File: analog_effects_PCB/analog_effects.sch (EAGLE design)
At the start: 79 parts, among them J1 RN111PC, J2 SP-3533-02, J3 SAMTEC-SSQ-120-01-X-DJ, U1 TL082, U10 TS5A3359DCUT, U11 TS5A3359DCUT, U12 TS5A3359DCUT, U13 TS5A3359DCUT, U14 TS5A3359DCUT, U2 AD5241BRZ1M, U4 AD5241BRZ100, U7 AD5258BRMZ1-R7, U8 AD5241BRZ1M, U9 TS5A3359DCUT

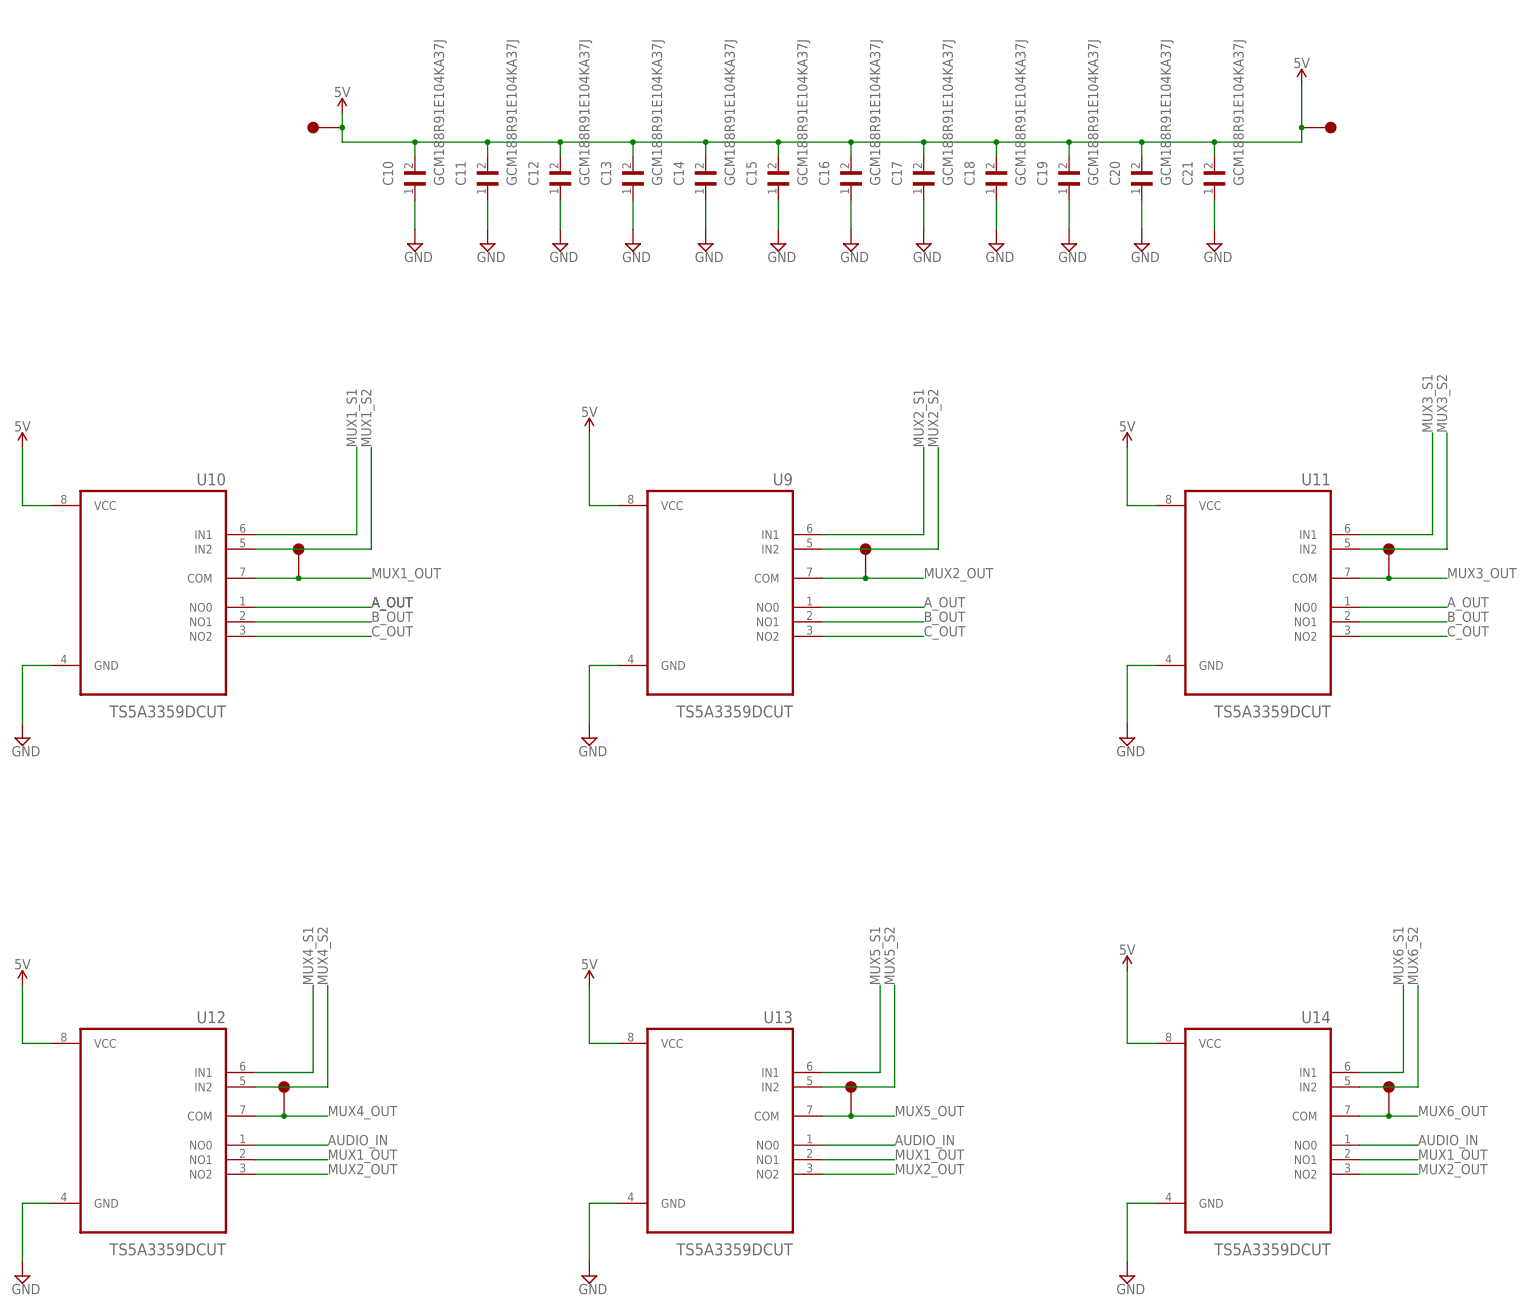
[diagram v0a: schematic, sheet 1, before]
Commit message: Adding all files that were needed, Capstone is completed and it worked
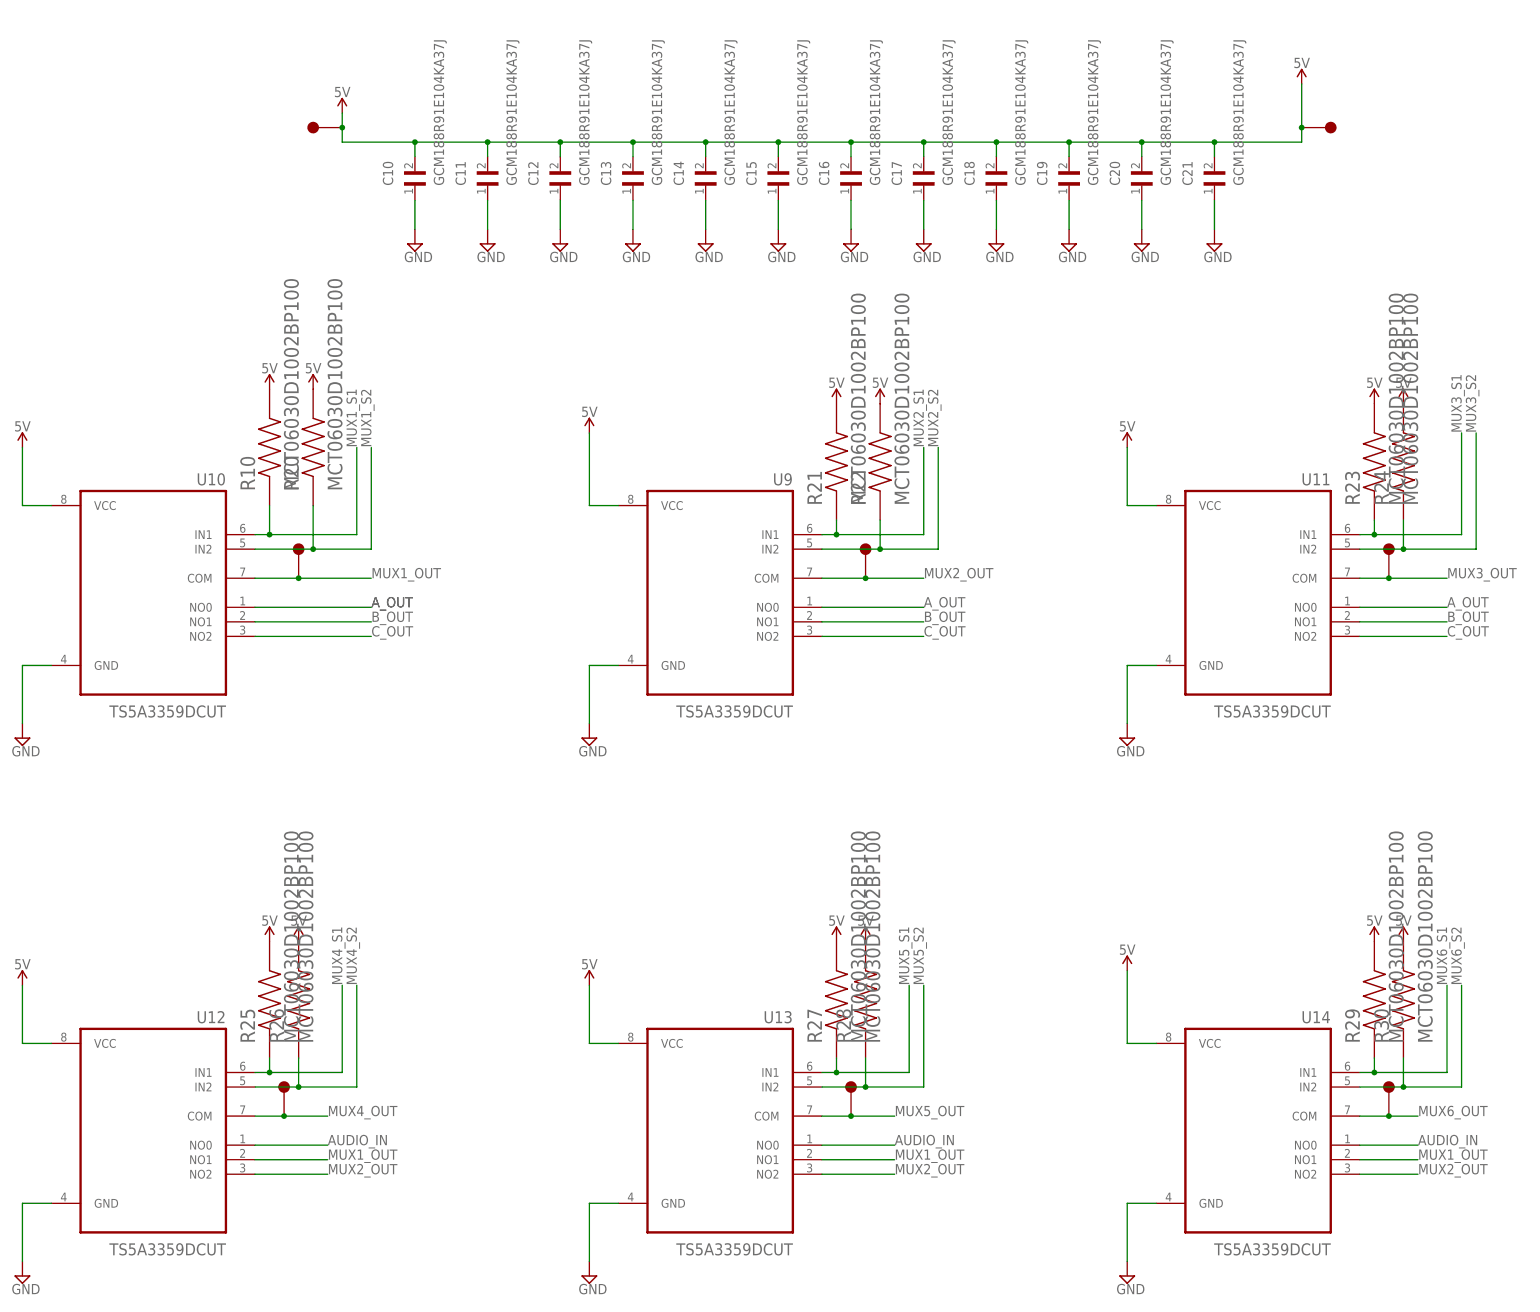
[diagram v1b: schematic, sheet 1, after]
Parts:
- removed BT1, BT2: BC9VPC, BC9VPC:BC9VPC
- removed J2: SP-3533-02, SP-3533-02:SP-3533-02
- added J4: SJ-3523-SMT-TR, SJ-3523-SMT-TR:SJ-3523-SMT-TR
- added R10, R20, R21, R22, R23, R24, R25, R26, R27, R28, R29, R30: MCT06030D1002BP100, MCT06030D1002BP100:MCT06030D1002BP100
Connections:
- removed net N$11: BT2.-, R17.2, R19.2, TP9.TP
- new net 9V_N: C4.2, C7.2, R17.2, R19.2, R5.1, TP2.TP, TP9.TP
- net 5V: now also R10.2, R20.2, R21.2, R22.2, R23.2, R24.2, R25.2, R26.2, R27.2, R28.2, R29.2, R30.2
- net GND: now also J4.1; no longer BT1.-, C4.2, C7.2, J2.S, R5.1, TP2.TP
- net MUX1_S1: now also R10.1
- net MUX1_S2: now also R20.1
- net MUX2_S1: now also R21.1
- net MUX2_S2: now also R22.1
- net MUX3_S1: now also R23.1
- net MUX3_S2: now also R24.1
- net MUX4_S1: now also R25.1
- net MUX4_S2: now also R26.1
- net MUX5_S1: now also R27.1
- net MUX5_S2: now also R28.1
- net MUX6_OUT: now also J4.2, J4.3; no longer J2.R, J2.T
- net MUX6_S1: now also R29.1
- net MUX6_S2: now also R30.1
- net N$1: no longer BT1.+
